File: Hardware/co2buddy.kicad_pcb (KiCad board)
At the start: 2 copper layers, 40.6 x 92.6 mm, 17 parts, among them J1 SERIAL, J2 USB_B_Micro, SW1 ENABLE, SW2 FLASH, U1 MH-Z19, U2 TLV75533PDBV, U3 ESP32-WROOM-32D

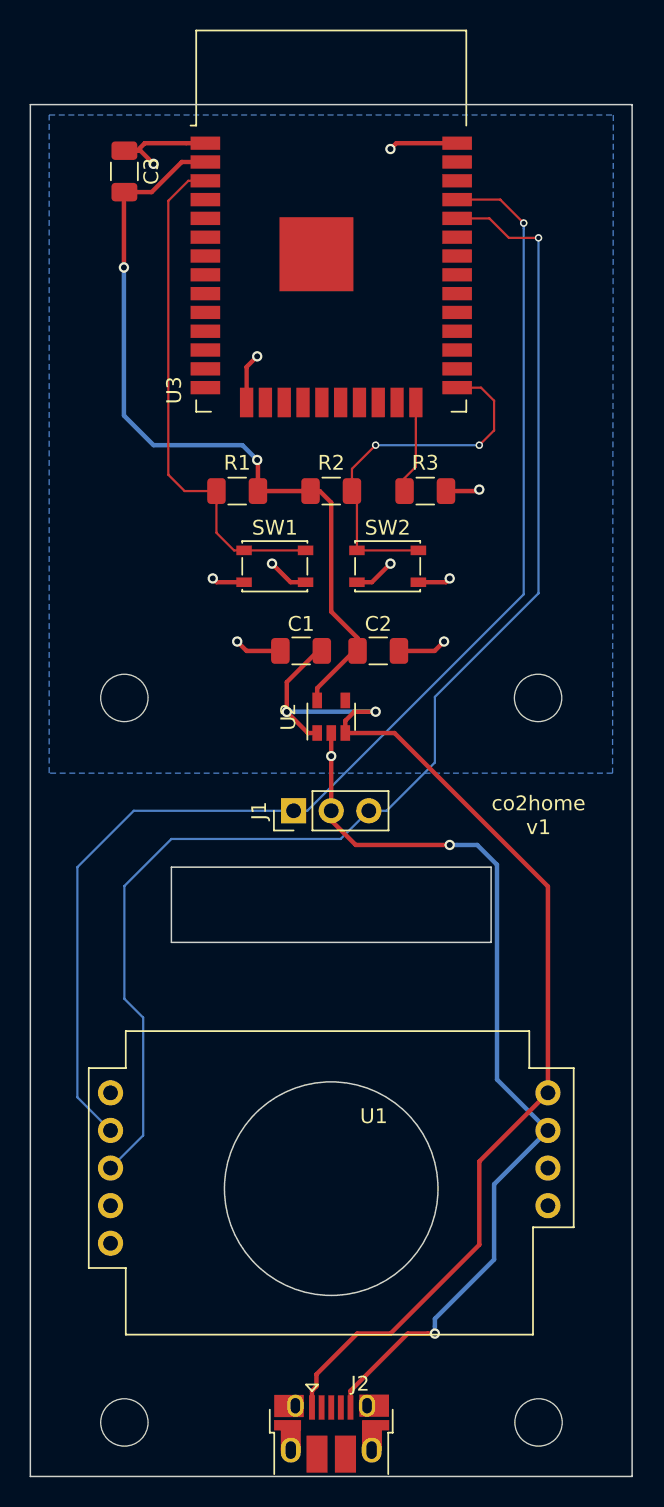
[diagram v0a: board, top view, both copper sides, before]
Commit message: v2
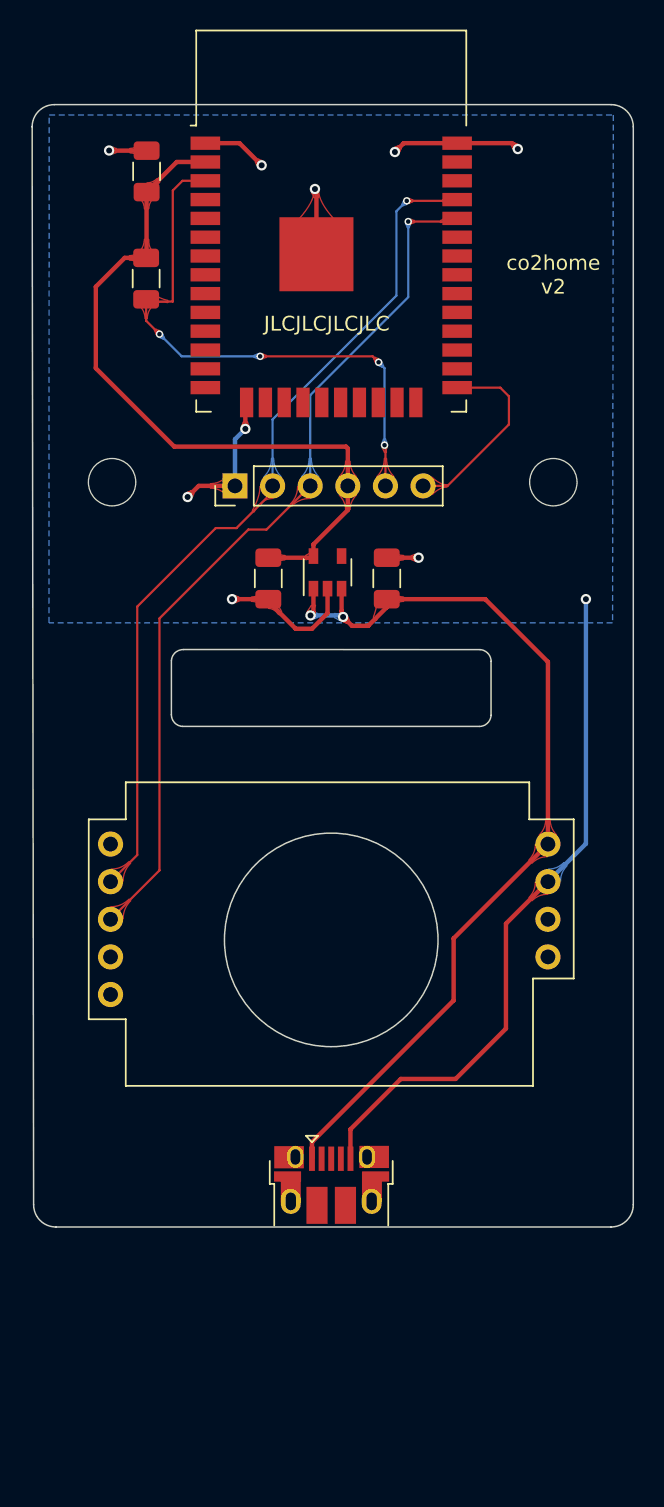
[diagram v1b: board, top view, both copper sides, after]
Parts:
- removed R2, R3: 100k, Resistor_SMD:R_1206_3216Metric
- removed the REF** at (121.1, 119.4)
- removed the REF** at (149.0, 119.4)
- removed the REF** at (121.1, 70.5)
- removed the REF** at (149.0, 70.5)
- removed SW1: ENABLE, Button_Switch_SMD:SW_SPST_PTS810
- removed SW2: FLASH, Button_Switch_SMD:SW_SPST_PTS810
- added REF**: MountingHole_3.2mm_M3, MountingHole:MountingHole_3.2mm_M3, F.Cu at (120.2, 55.9)
- added REF**: MountingHole_3.2mm_M3, MountingHole:MountingHole_3.2mm_M3, F.Cu at (150.0, 55.9)
- J1: value SERIAL -> esp32buddy; footprint Connector_PinHeader_2.54mm:PinHeader_1x03_P2.54mm_Vertical -> Connector_PinHeader_2.54mm:PinHeader_1x06_P2.54mm_Vertical
- J2: footprint Connector_USB:USB_Micro-B_Amphenol_10103594-0001LF_Horizontal -> !Greg:USB_Micro-B_Amphenol_10103594-0001LF_Horizontal
- moved J1 22.3 mm to (128.5, 56.1)
- moved J2 16.8 mm to (135.1, 103.4)
- moved U1 16.8 mm to (137.9, 85.4)
- moved R1 15.6 mm to (122.5, 42.1), turned to 90 degrees
- moved U2 9.75 mm to (134.8, 62.0)
- moved C2 8.89 mm to (130.8, 62.4), turned to 270 degrees
- moved C1 7.58 mm to (138.8, 62.4), turned to 270 degrees
- moved C3 1.50 mm to (122.6, 34.9)
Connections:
- J1 pad 1: /TXD -> GND
- J1 pad 2: GND -> /TXD
- R1 pad 1: Net-(R1-Pad1) -> /EN
- U3 pad 24: Net-(R3-Pad1) -> (no net)
- U3 pad 25: Net-(R2-Pad1) -> /GPIO0
- U3 pad 3: Net-(R1-Pad1) -> /EN
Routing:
- net /EN: track 0.00 -> 38.7 mm, vias 0 -> 4
- net Net-(R1-Pad1): track 34.6 -> 0.00 mm
- net /RXD: track 89.3 -> 59.6 mm
- net /TXD: track 86.7 -> 58.5 mm
- net Net-(R2-Pad1): track 25.3 -> 0.00 mm, vias 2 -> 0
- net VBUS: track 78.1 -> 63.1 mm
- net /GPIO0: track 0.00 -> 13.2 mm
- net GND: track 98.0 -> 87.8 mm, vias 13 -> 10
- net Net-(R3-Pad1): track 6.30 -> 0.00 mm
- net +3V3: track 54.4 -> 49.8 mm, vias 2 -> 0
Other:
- board size 40.6 x 92.6 mm -> 40.6 x 75.8 mm
- board text added: "JLCJLCJLCJLC"
- board text added: "co2home v2"
- board text removed: "co2home v1"
